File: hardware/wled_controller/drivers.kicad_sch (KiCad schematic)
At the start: 12 parts, among them J1 Screw_Terminal_01x03, J10 Screw_Terminal_01x03, J11 Screw_Terminal_01x03, J12 Screw_Terminal_01x03, J2 Screw_Terminal_01x03, J3 Screw_Terminal_01x03, J4 Screw_Terminal_01x03, J5 Screw_Terminal_01x03, J6 Screw_Terminal_01x03, J7 Screw_Terminal_01x03, J8 Screw_Terminal_01x03, J9 Screw_Terminal_01x03

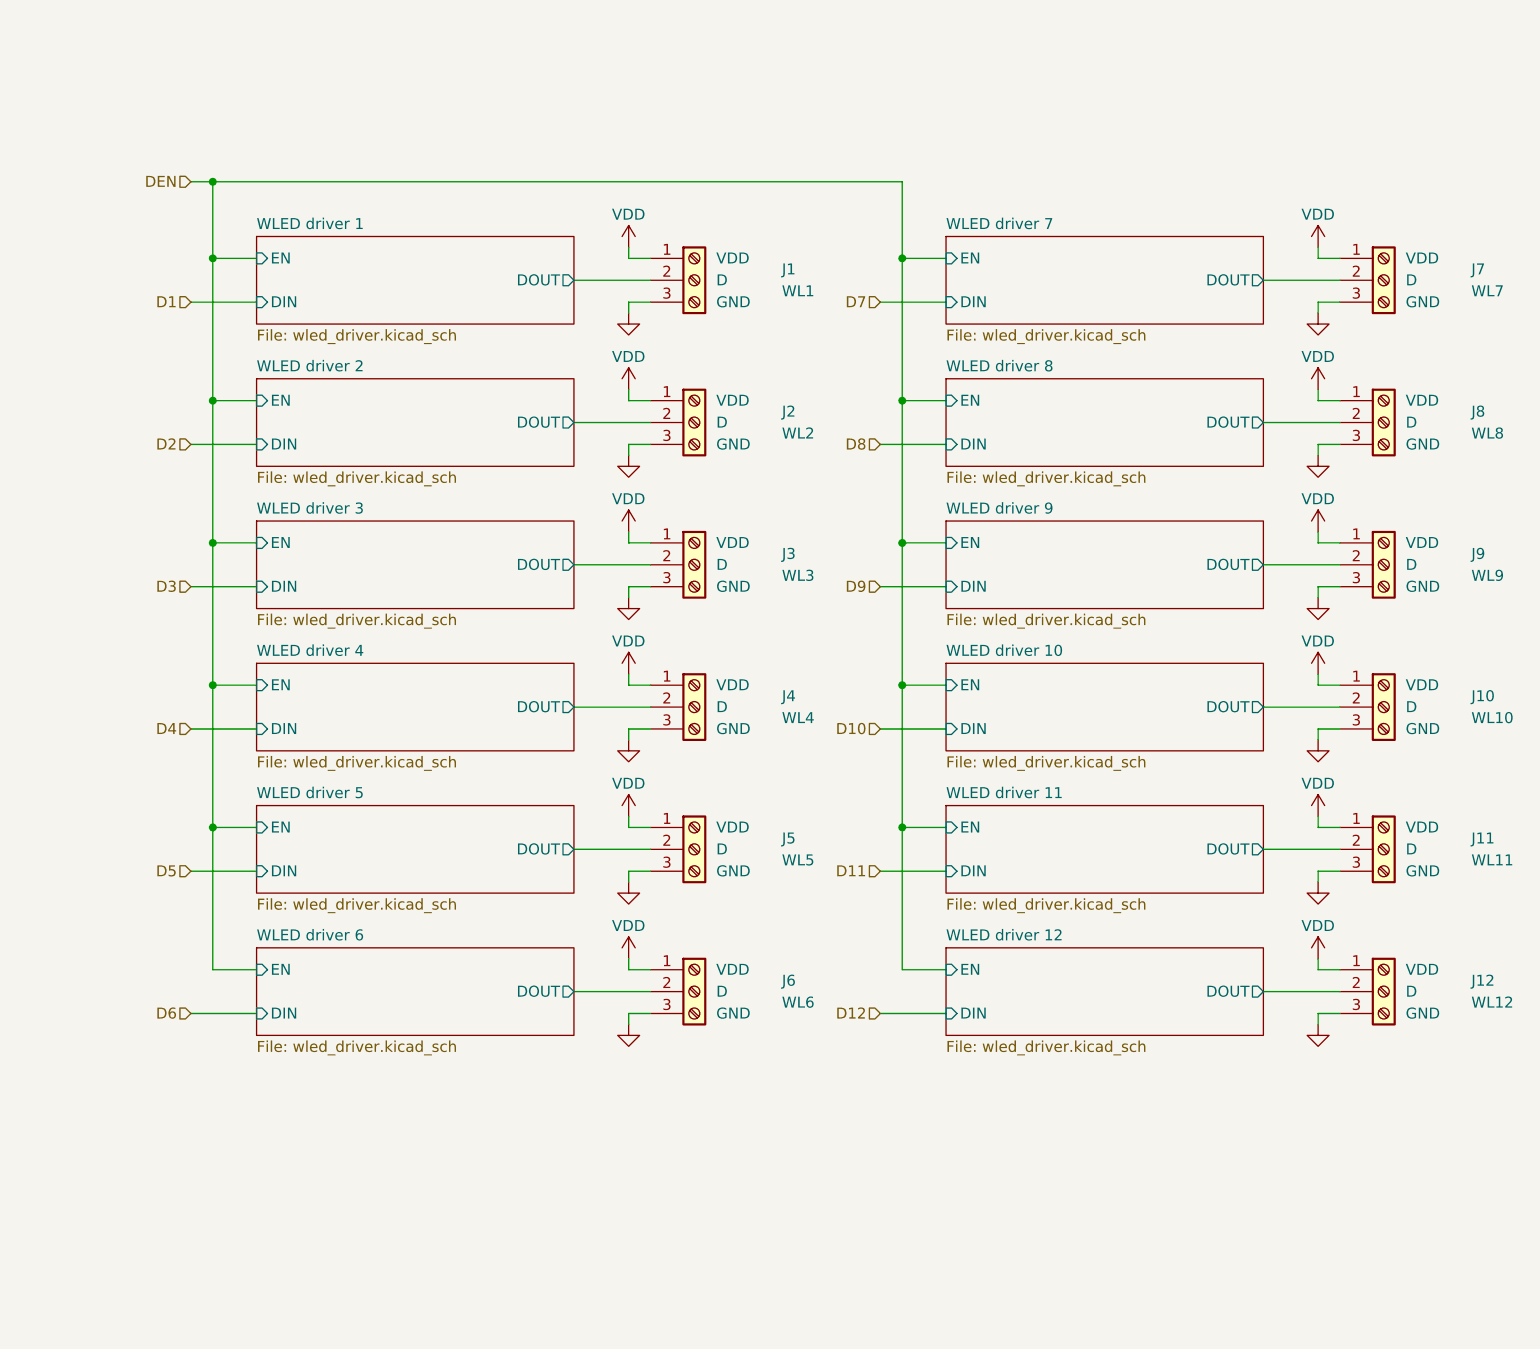
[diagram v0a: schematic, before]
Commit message: finalise schematic
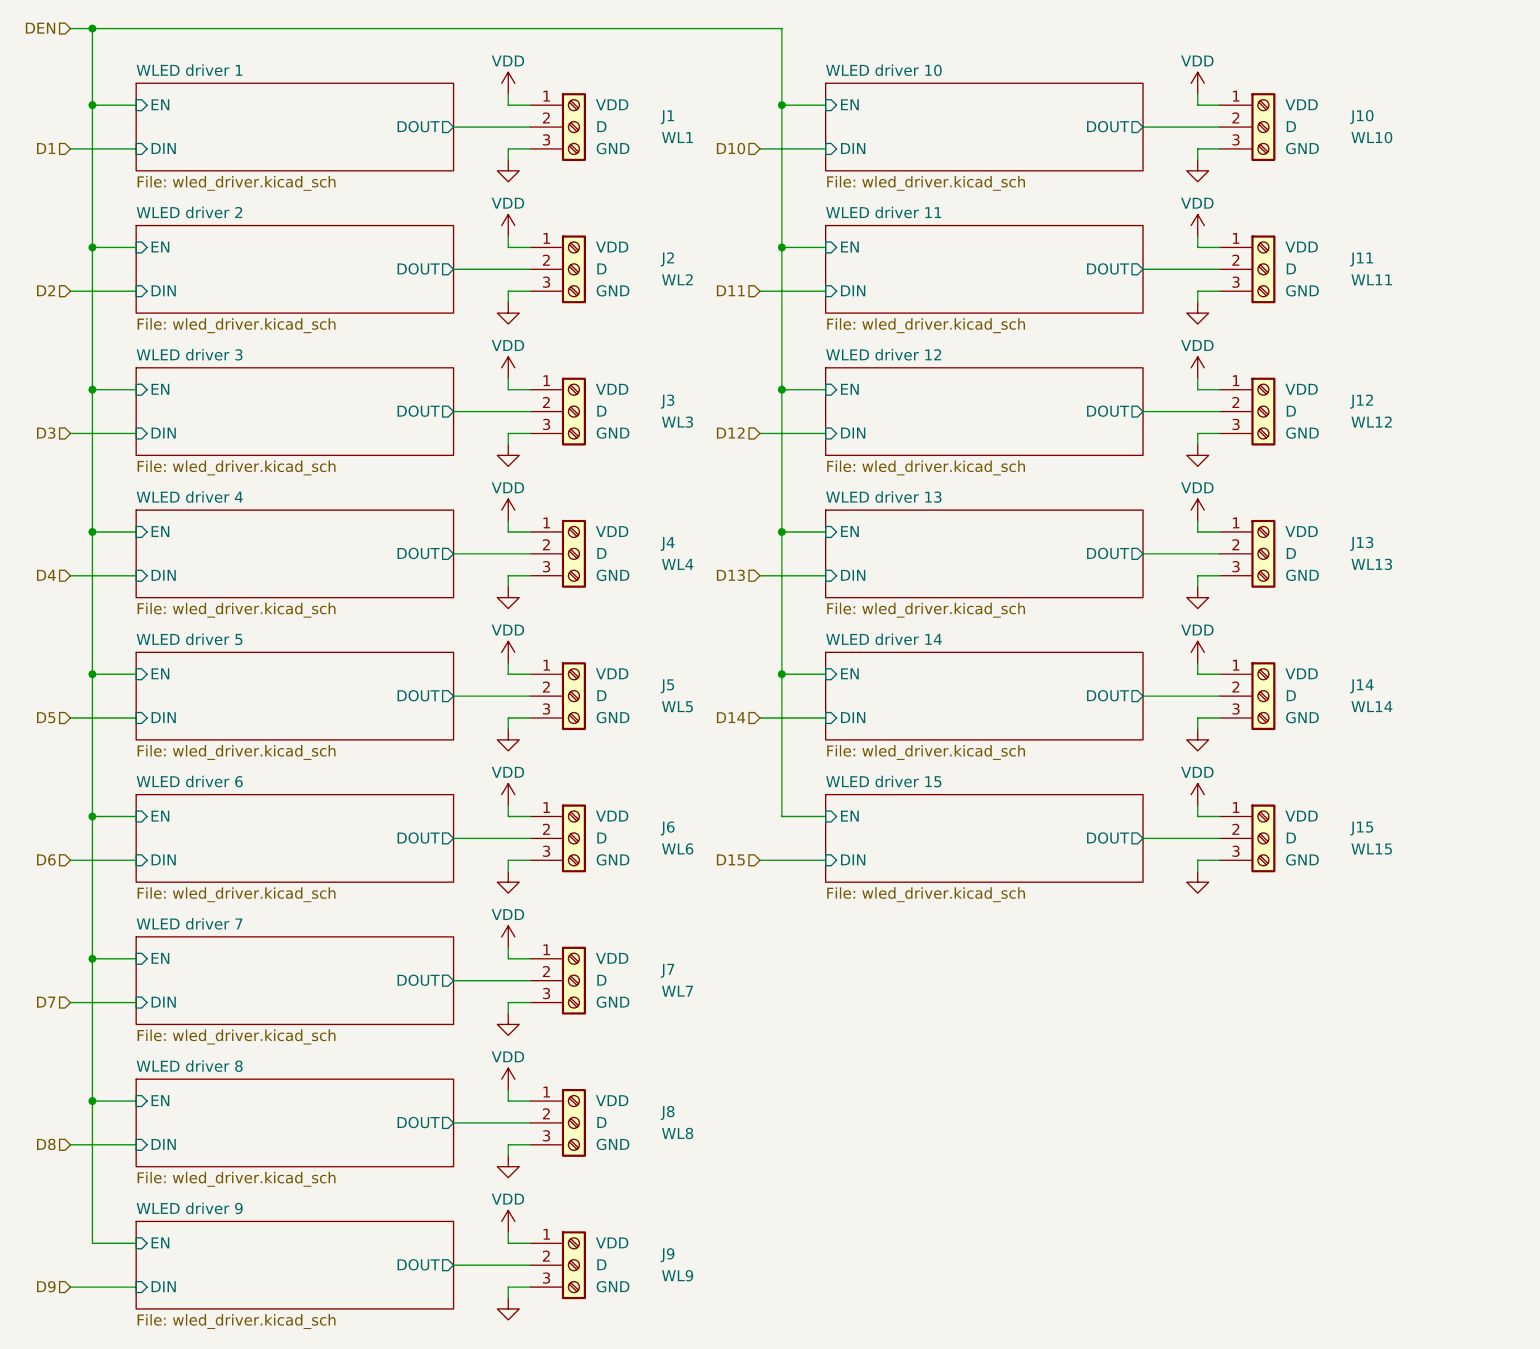
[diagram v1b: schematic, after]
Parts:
- added J13, J14, J15: Screw_Terminal_01x03, conn:TerminalBlock_4Ucon_1x03_P3.50mm_Vertical, symbol conn:Screw_Terminal_01x03
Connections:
- net GND: now also J13.3 (Pin_3), J14.3 (Pin_3), J15.3 (Pin_3)
- net VDD: now also J13.1 (Pin_1), J14.1 (Pin_1), J15.1 (Pin_1)
- new net WLED driver 13/DOUT: J13.2 (Pin_2)
- new net WLED driver 14/DOUT: J14.2 (Pin_2)
- new net WLED driver 15/DOUT: J15.2 (Pin_2)
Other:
- added sheet WLED driver 13 (wled_driver.kicad_sch)
- added sheet WLED driver 14 (wled_driver.kicad_sch)
- added sheet WLED driver 15 (wled_driver.kicad_sch)
- moved on the sheet: J1, J10, J11, J12, J2, J3, J4, J5, J6, J7, J8, J9
